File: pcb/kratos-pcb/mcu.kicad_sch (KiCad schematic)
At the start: 2 parts, among them SW1 SW_Push, U1 ESP32-DEVKIT-V1

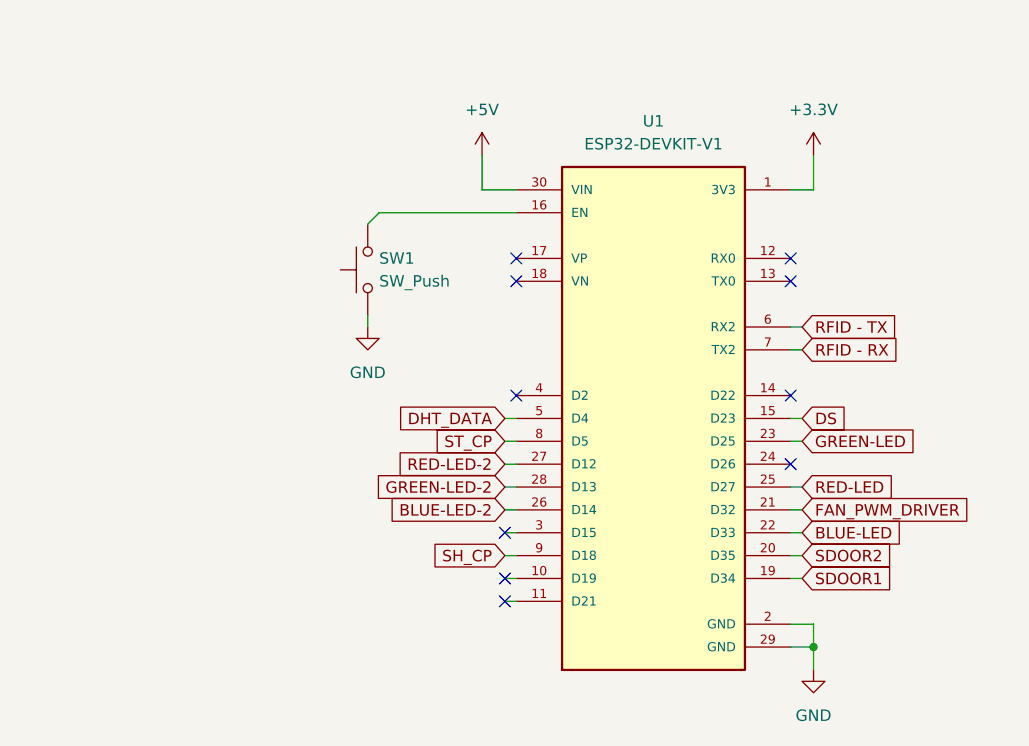
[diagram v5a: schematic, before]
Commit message: ### Modify
   - schematic
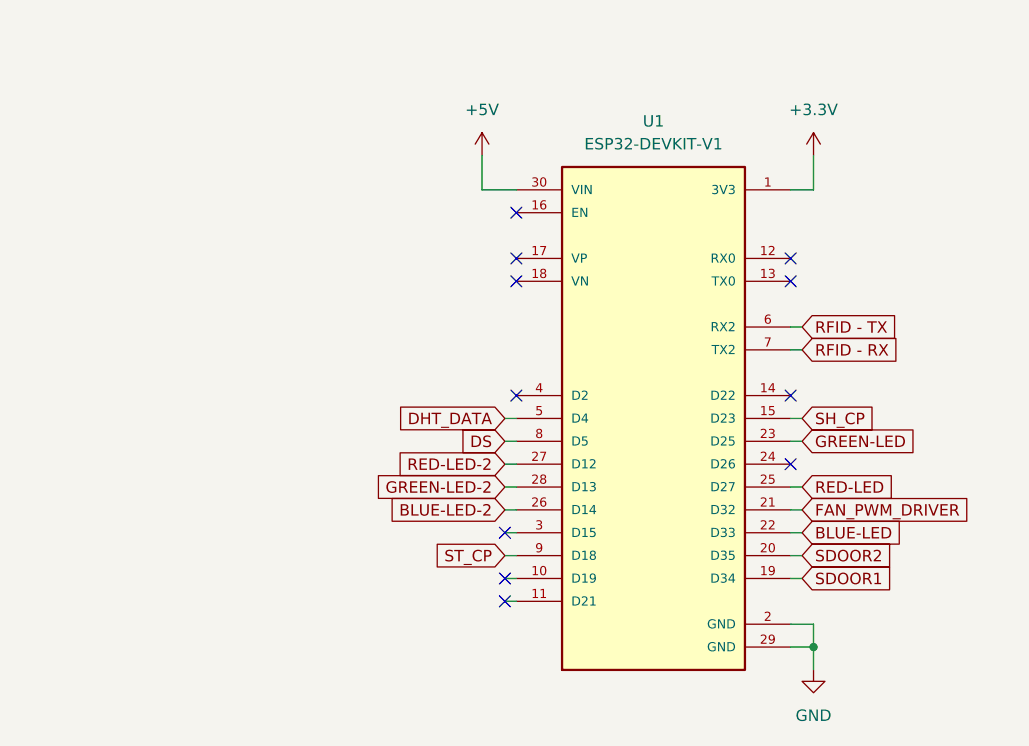
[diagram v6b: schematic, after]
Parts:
- removed SW1: SW_Push, Button_Switch_THT:SW_PUSH_6mm_H4.3mm, symbol Switch:SW_Push
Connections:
- net DS: now also U1.8 (D5); no longer U1.15 (D23)
- net SH_CP: now also U1.15 (D23); no longer U1.9 (D18)
- net ST_CP: now also U1.9 (D18); no longer U1.8 (D5)
- no-connect marks 10 -> 11
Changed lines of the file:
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@@
   (no_connect (at 127 116.84))
   (no_connect (at 158.75 78.74))
+  (no_connect (at 128.27 73.66))
   (no_connect (at 128.27 81.28))
   (wire (pts (xy 160.02 106.68) (xy 158.75 106.68))
@@
     (stroke (width 0) (type default))
   )
-  (wire (pts (xy 111.76 74.93) (xy 113.03 73.66))
-    (stroke (width 0) (type default))
-  )
   (wire (pts (xy 127 106.68) (xy 128.27 106.68))
     (stroke (width 0) (type default))
@@
   )
   (wire (pts (xy 127 104.14) (xy 128.27 104.14))
-    (stroke (width 0) (type default))
-  )
-  (wire (pts (xy 128.27 73.66) (xy 113.03 73.66))
-    (stroke (width 0) (type default))
-  )
-  (wire (pts (xy 111.76 85.09) (xy 111.76 86.36))
     (stroke (width 0) (type default))
   )
@@
     )
   )
-  (global_label "SH_CP" (shape input) (at 127 111.76 180) (fields_autoplaced)
-    (effects (font (size 1.27 1.27)) (justify right))
-    (property "Intersheetrefs" "${INTERSHEET_REFS}" (at 117.9672 111.76 0)
-      (effects (font (size 1.27 1.27)) (justify right) hide)
+  (global_label "SH_CP" (shape input) (at 160.02 96.52 0) (fields_autoplaced)
+    (effects (font (size 1.27 1.27)) (justify left))
+    (property "Intersheetrefs" "${INTERSHEET_REFS}" (at 169.0528 96.52 0)
+      (effects (font (size 1.27 1.27)) (justify left) hide)
     )
   )
@@
     (property "Intersheetrefs" "${INTERSHEET_REFS}" (at 171.7137 104.14 0)
       (effects (font (size 1.27 1.27)) (justify left) hide)
+    )
+  )
+  (global_label "ST_CP" (shape input) (at 127 111.76 180) (fields_autoplaced)
+    (effects (font (size 1.27 1.27)) (justify right))
+    (property "Intersheetrefs" "${INTERSHEET_REFS}" (at 118.3301 111.76 0)
+      (effects (font (size 1.27 1.27)) (justify right) hide)
     )
   )
@@
     )
   )
-  (global_label "ST_CP" (shape input) (at 127 99.06 180) (fields_autoplaced)
+  (global_label "DS" (shape input) (at 127 99.06 180) (fields_autoplaced)
     (effects (font (size 1.27 1.27)) (justify right))
-    (property "Intersheetrefs" "${INTERSHEET_REFS}" (at 118.3301 99.06 0)
+    (property "Intersheetrefs" "${INTERSHEET_REFS}" (at 121.5353 99.06 0)
       (effects (font (size 1.27 1.27)) (justify right) hide)
     )
@@
     (effects (font (size 1.27 1.27)) (justify left))
     (property "Intersheetrefs" "${INTERSHEET_REFS}" (at 173.2257 88.9 0)
-      (effects (font (size 1.27 1.27)) (justify left) hide)
-    )
-  )
-  (global_label "DS" (shape input) (at 160.02 96.52 0) (fields_autoplaced)
-    (effects (font (size 1.27 1.27)) (justify left))
-    (property "Intersheetrefs" "${INTERSHEET_REFS}" (at 165.4847 96.52 0)
       (effects (font (size 1.27 1.27)) (justify left) hide)
     )
@@
         )
       )
-    )
-  )
-  (symbol (lib_id "Switch:SW_Push") (at 111.76 80.01 90) (unit 1)
-    (in_bom yes) (on_board yes) (dnp no) (fields_autoplaced)
-    (property "Reference" "SW1" (at 113.03 78.74 90)
-      (effects (font (size 1.27 1.27)) (justify right))
-    )
-    (property "Value" "SW_Push" (at 113.03 81.28 90)
-      (effects (font (size 1.27 1.27)) (justify right))
-    )
-    (property "Footprint" "Button_Switch_THT:SW_PUSH_6mm_H4.3mm" (at 106.68 80.01 0)
-      (effects (font (size 1.27 1.27)) hide)
-    )
-    (property "Datasheet" "~" (at 106.68 80.01 0)
-      (effects (font (size 1.27 1.27)) hide)
-    )
-    (pin "1")
-    (pin "2")
-    (instances
-      (project "kratos-pcb"
-        (path "/12f1b997-8c5f-4ef7-b036-7873ddaba48e/6278edd7-c4ea-4e2d-a20d-bed0b1d88716"
-          (reference "SW1") (unit 1)
-        )
-      )
-    )
-  )
-  (symbol (lib_id "power:GND") (at 111.76 86.36 0) (unit 1)
-    (in_bom yes) (on_board yes) (dnp no) (fields_autoplaced)
-    (property "Reference" "#PWR09" (at 111.76 92.71 0)
-      (effects (font (size 1.27 1.27)) hide)
-    )
-    (property "Value" "GND" (at 111.76 91.44 0)
-      (effects (font (size 1.27 1.27)))
-    )
-    (property "Footprint" "" (at 111.76 86.36 0)
-      (effects (font (size 1.27 1.27)) hide)
-    )
-    (property "Datasheet" "" (at 111.76 86.36 0)
-      (effects (font (size 1.27 1.27)) hide)
-    )
-    (pin "1")
-    (instances
-      (project "kratos-pcb"
-        (path "/12f1b997-8c5f-4ef7-b036-7873ddaba48e/6278edd7-c4ea-4e2d-a20d-bed0b1d88716"
-          (reference "#PWR09") (unit 1)
-        )
-      )
